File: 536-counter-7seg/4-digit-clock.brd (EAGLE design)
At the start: 100 x 100 mm, 36 parts, among them IC1 SLG46826GTR, IC2 SLG46826GTR, IC3 SLG46826GTR, IC4 SLG46826GTR, IC5 SLG46826GTR, IC7 SLG46826GTR

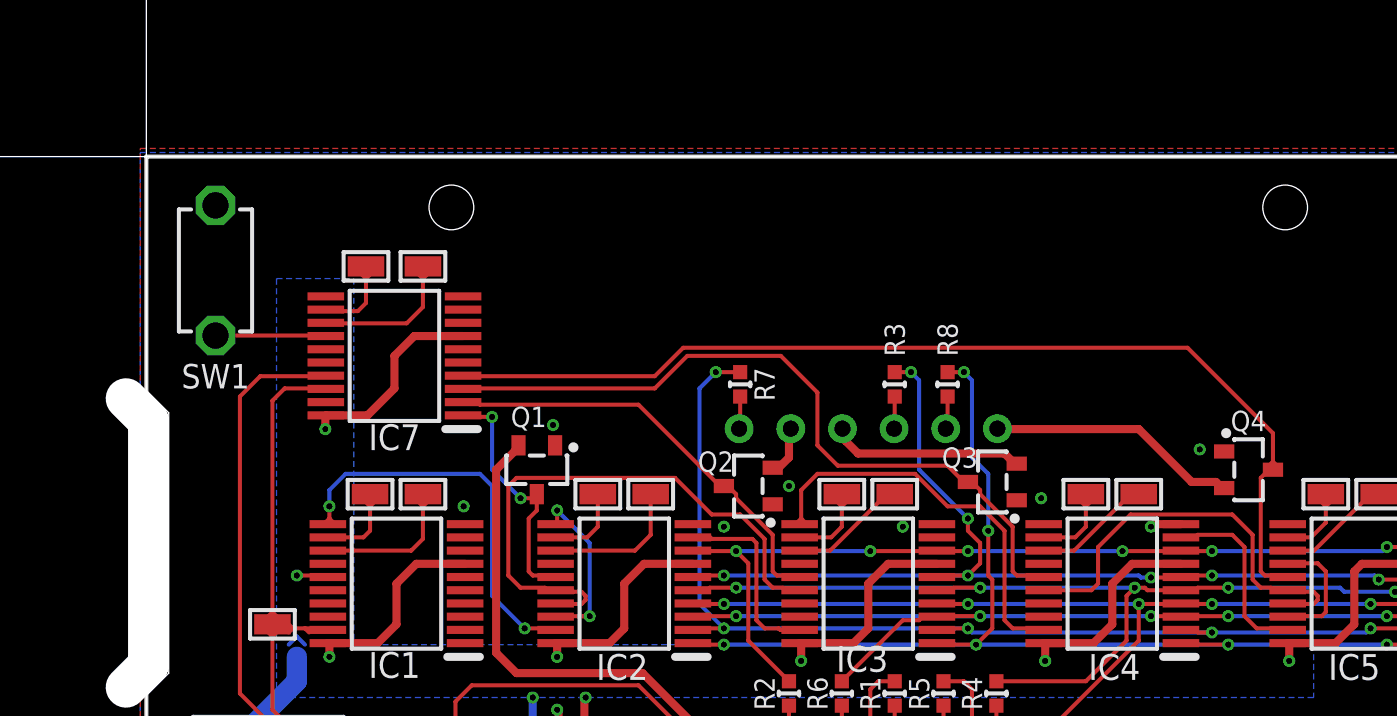
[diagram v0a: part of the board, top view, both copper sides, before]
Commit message: update pcb layouts
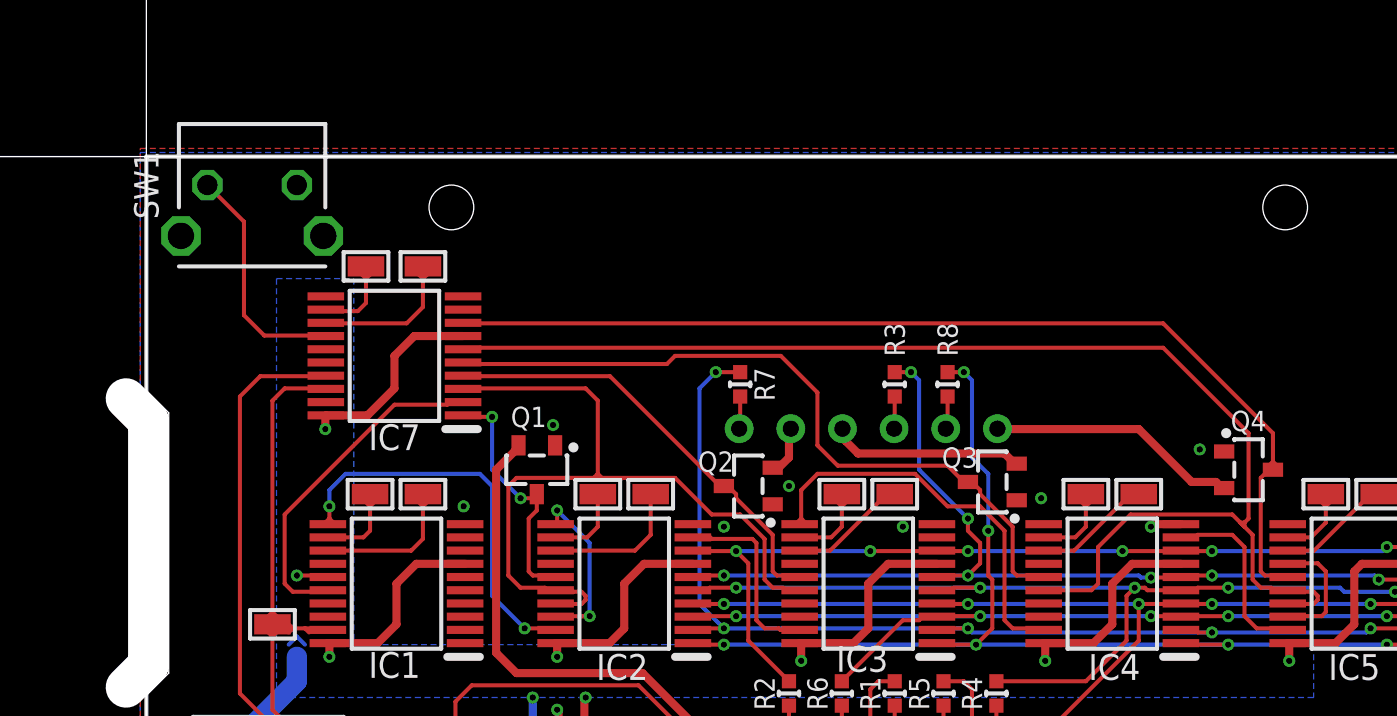
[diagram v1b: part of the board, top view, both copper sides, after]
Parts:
- SW1: device mylib:SW-TACTSW-P8073 -> mylib:SW-TACTSW-TL1105S
- moved SW1 4.57 mm to (19.2, 44.6), turned to 180 degrees
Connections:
- new net N$51: IC1.16, IC7.2
- net GND: now also SW1.1; no longer SW1.A1
- net N$17: now also IC7.4; no longer IC7.2
- net N$18: now also IC7.5; no longer IC7.3
- net N$22: now also IC7.8; no longer IC7.4
- net N$26: now also IC7.3
- net N$27: now also IC7.6
- net N$49: now also SW1.2; no longer SW1.A2
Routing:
- net N$27: track 20.8 -> 66.2 mm
- net N$51: track 0.00 -> 16.8 mm
- net N$26: track 28.3 -> 39.6 mm
- net N$49: track 5.44 -> 11.6 mm
- net N$17: track 21.3 -> 21.8 mm
